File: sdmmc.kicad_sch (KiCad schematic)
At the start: 18 parts, among them U15 MLD-TF PUSH-H18

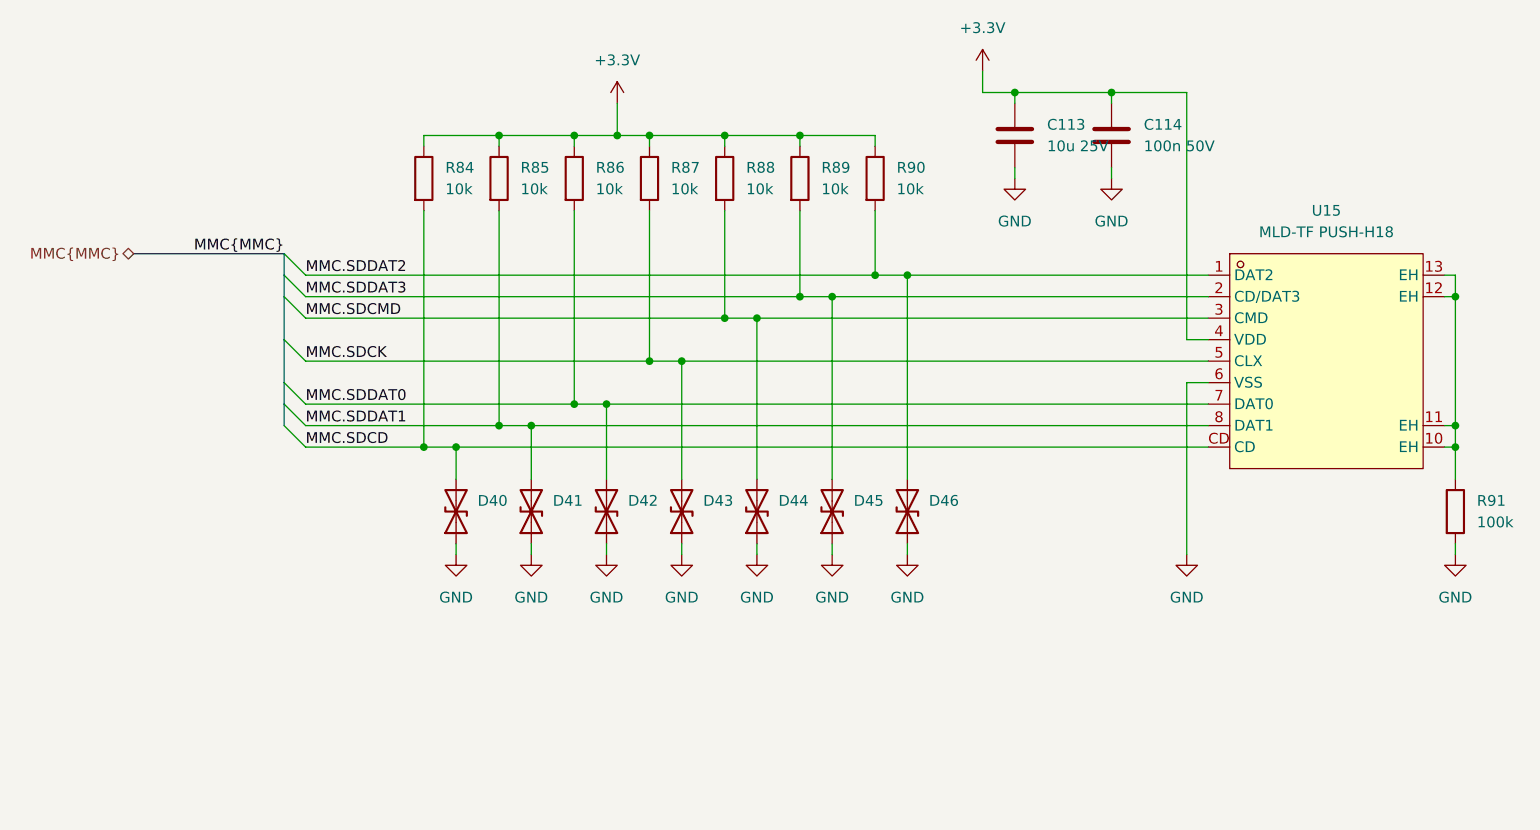
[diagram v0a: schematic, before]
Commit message: bunch of stuff
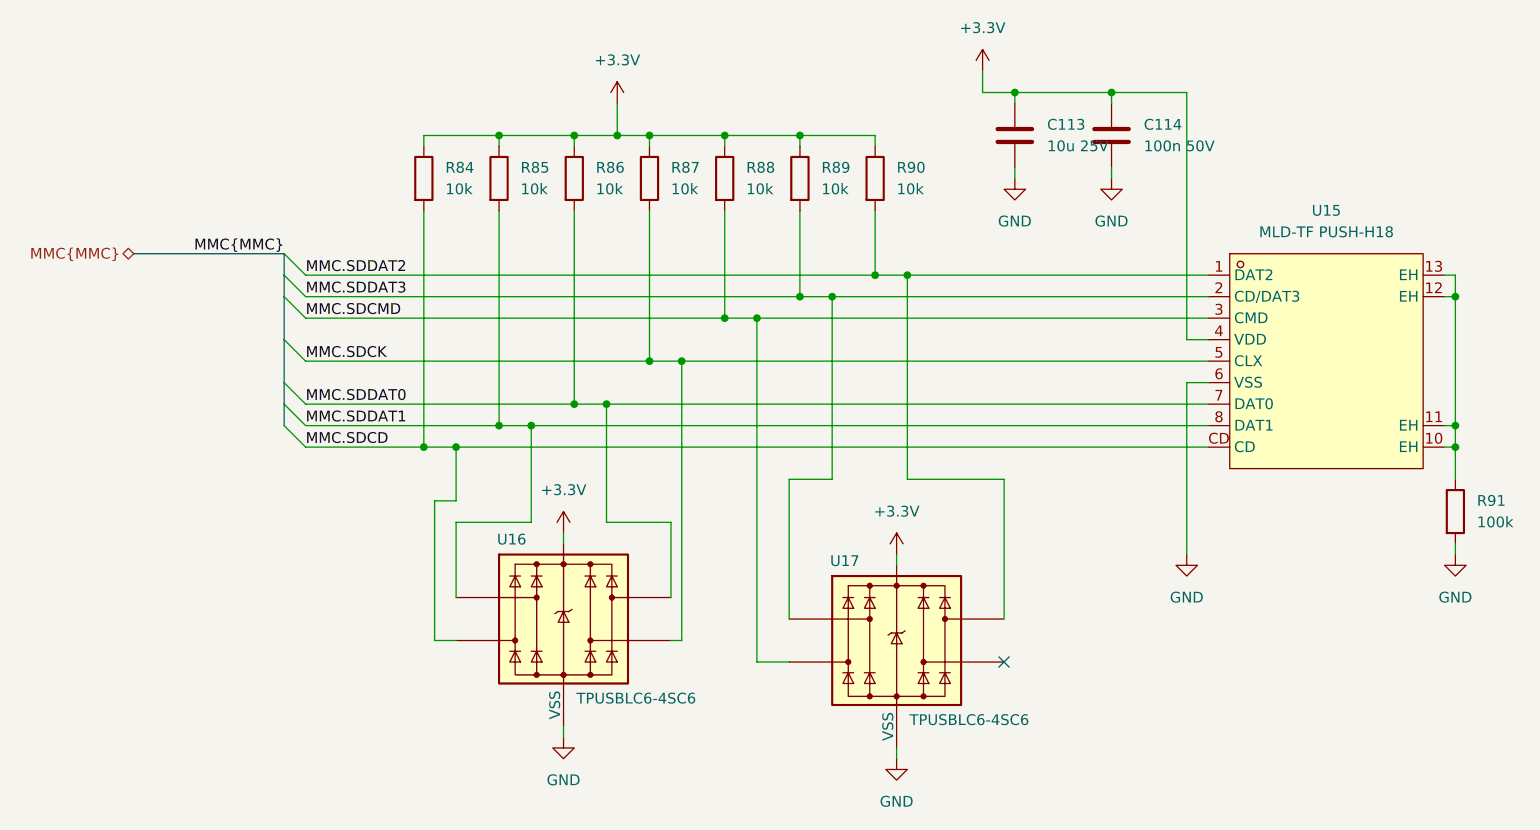
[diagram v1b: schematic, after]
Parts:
- removed D40, D41, D42, D43, D44, D45, D46: D_TVS, symbol Device:D_TVS
- added U16, U17: TPUSBLC6-4SC6, Package_TO_SOT_SMD:SOT-23-6_Handsoldering, symbol Library:TPUSBLC6-4SC6
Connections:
- net +3.3V: now also U16.5, U17.5
- net GND: now also U16.2 (VSS), U17.2 (VSS)
- net MMC.SDCD: now also U16.1
- net MMC.SDCK: now also U16.3
- net MMC.SDCMD: now also U17.1
- net MMC.SDDAT0: now also U16.4
- net MMC.SDDAT1: now also U16.6
- net MMC.SDDAT2: now also U17.4
- net MMC.SDDAT3: now also U17.6
- no-connect marks 0 -> 1
